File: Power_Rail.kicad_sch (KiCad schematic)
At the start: 16 parts, among them J2 USB_C_Receptacle_USB2.0_16P, U3 AMS1117

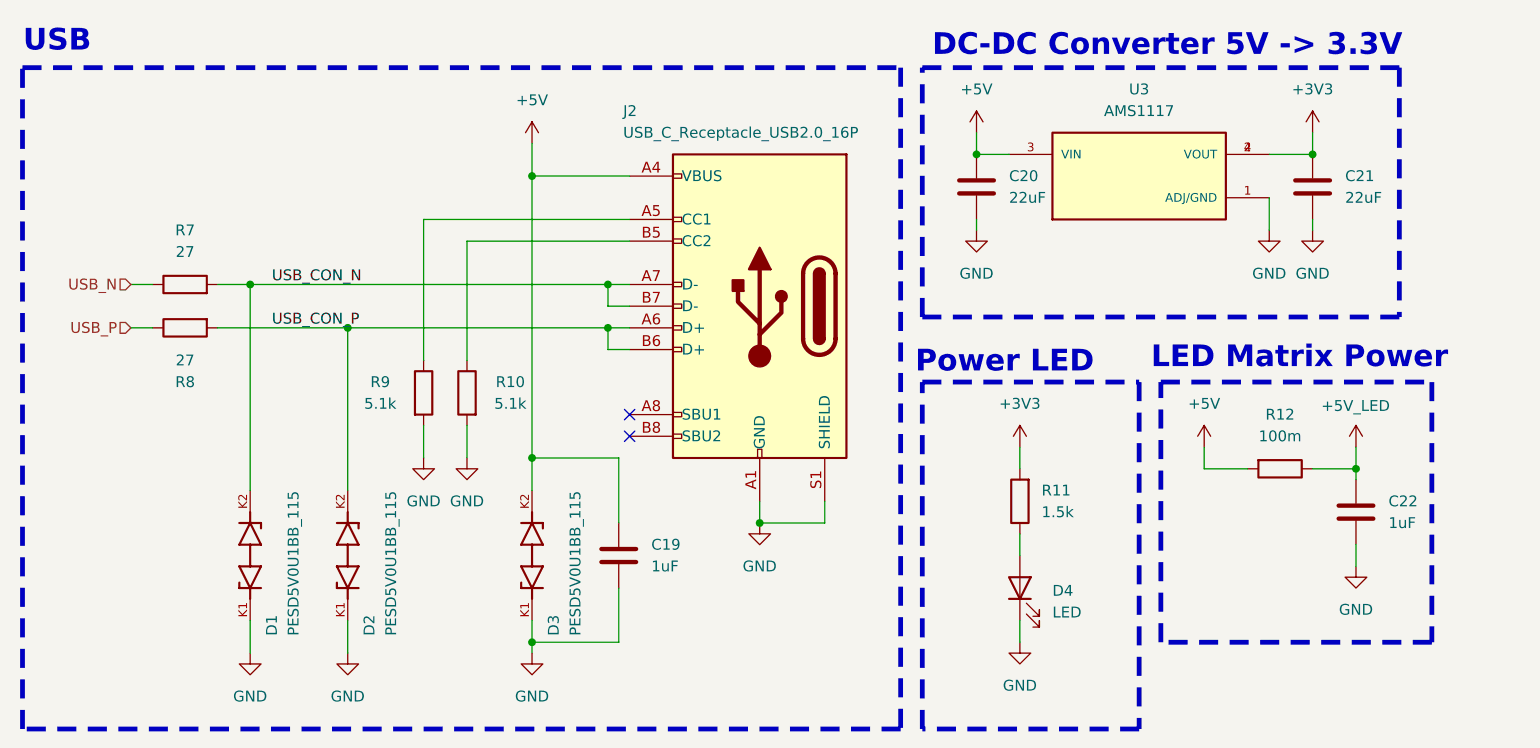
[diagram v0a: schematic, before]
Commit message: Schematic Clean Up
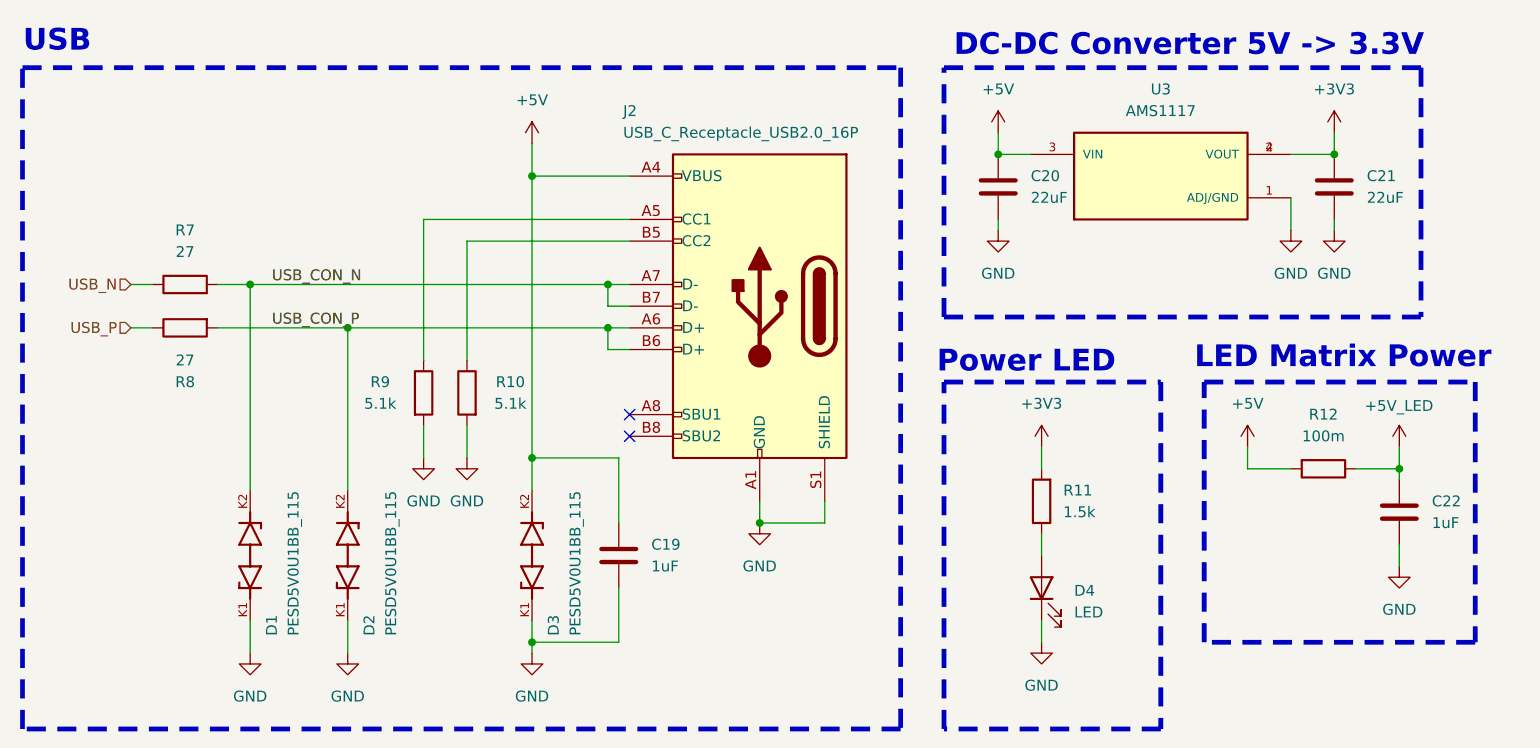
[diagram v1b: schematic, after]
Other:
- moved on the sheet: C20, C21, C22, D4, R11, R12, U3

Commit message: PCB Update
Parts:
- J2: footprint Connector_USB:USB_C_Receptacle_GCT_USB4105-xx-A_16P_TopMnt_Horizontal -> Connector_USB:USB_C_Receptacle_HRO_TYPE-C-31-M-12
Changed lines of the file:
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@@
 			)
 		)
-		(property "Footprint" "Connector_USB:USB_C_Receptacle_GCT_USB4105-xx-A_16P_TopMnt_Horizontal"
+		(property "Footprint" "Connector_USB:USB_C_Receptacle_HRO_TYPE-C-31-M-12"
 			(at 97.79 45.72 0)
 			(effects
